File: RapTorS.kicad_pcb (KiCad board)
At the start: 2 copper layers, 22 parts, among them J1 Molex 48037-2200, J2 TestPoint, J3 TestPoint, J4 TestPoint, J5 TestPoint, J6 TestPoint, U1 PIC16LF1454-I_ML, U2 TLV71333PDBV, U3 E07-M1101S

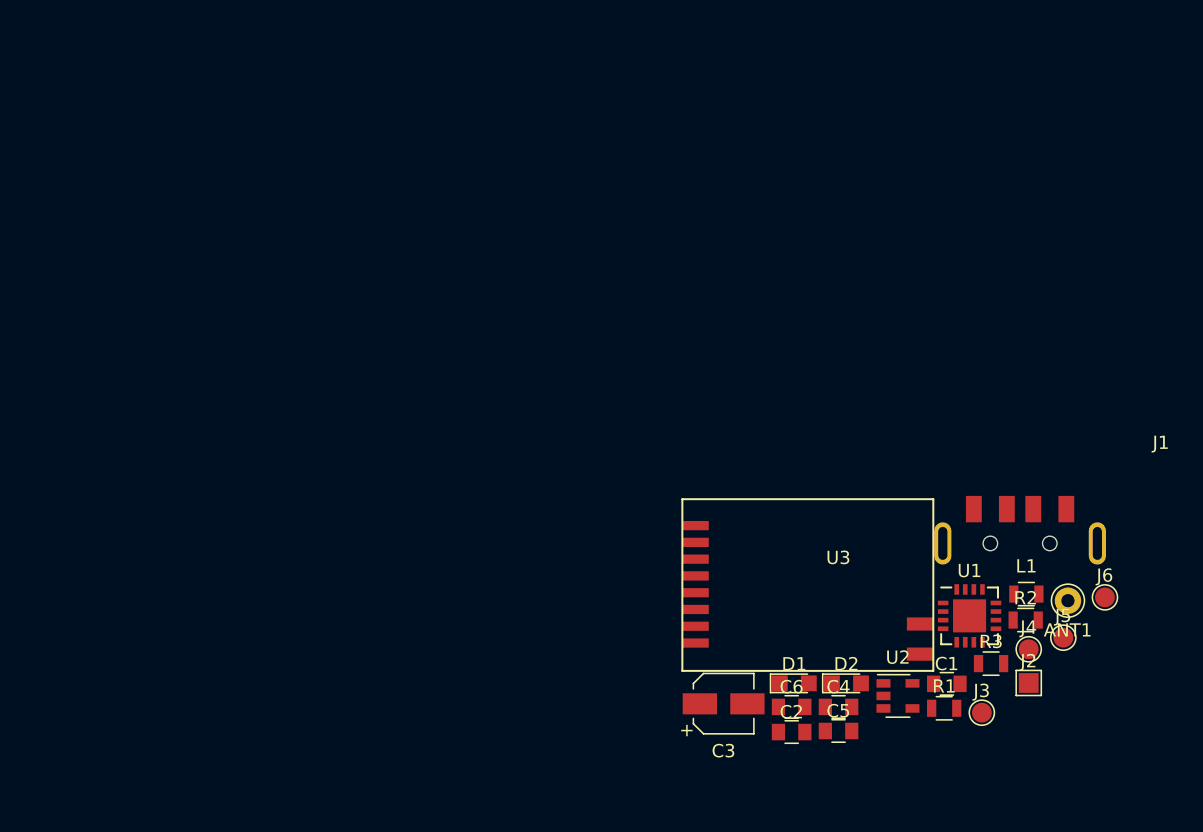
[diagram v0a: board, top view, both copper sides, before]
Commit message: first placement
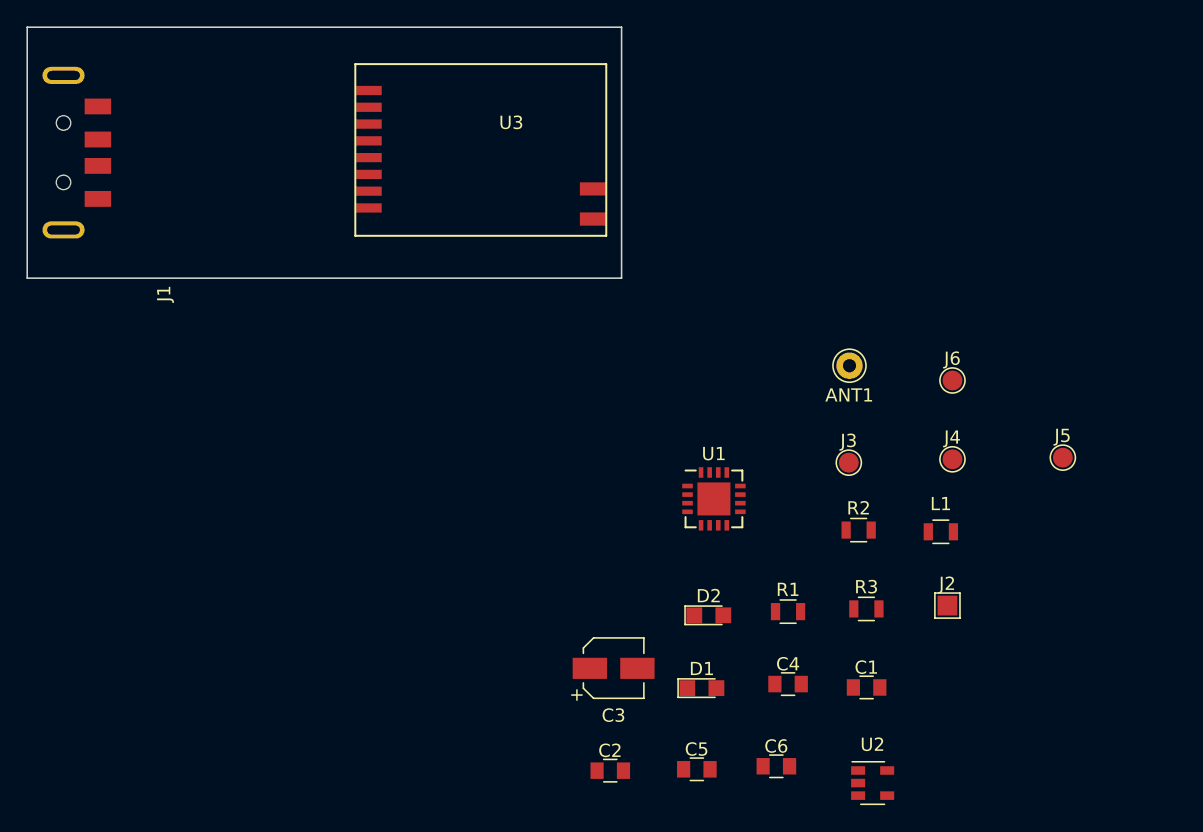
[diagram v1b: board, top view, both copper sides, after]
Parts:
- moved J1 78.2 mm to (2.75, 9.50), turned to 270 degrees
- moved U3 41.2 mm to (24.8, 2.79)
- moved ANT1 24.3 mm to (62.3, 25.6)
- moved J3 21.4 mm to (62.2, 33.0)
- moved U1 21.3 mm to (52.0, 35.7)
- moved J6 20.1 mm to (70.1, 26.7)
- moved J4 15.5 mm to (70.1, 32.7)
- moved R2 14.4 mm to (63.0, 38.1)
- moved C2 14.0 mm to (44.1, 56.3)
- moved R1 13.9 mm to (57.6, 44.2)
- moved J5 13.6 mm to (78.4, 32.6)
- moved D2 11.6 mm to (51.6, 44.5)
- moved C5 11.1 mm to (50.7, 56.2)
- moved R3 10.3 mm to (63.5, 44.0)
- moved C3 8.75 mm to (44.4, 48.5)
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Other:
- board outline added: 45 x 19 mm
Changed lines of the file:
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@@
   (general
     (thickness 1.6)
-    (drawings 0)
+    (drawings 4)
     (tracks 0)
     (zones 0)
@@
     (pad_to_mask_clearance 0.2)
     (aux_axis_origin 0 0)
-    (visible_elements FFFFFF7F)
+    (visible_elements FEFFF77F)
     (pcbplotparams
       (layerselection 0x010fc_ffffffff)
@@
   )
   (module Capacitors_SMD:CP_Elec_4x4.5 (layer F.Cu)
-    (at 52.727201 51.228801)
+    (at 44.3992 48.5394)
     (descr "SMT capacitor, aluminium electrolytic, 4x4.5")
     (attr smd)
@@
   )
   (module Capacitors_SMD:C_0805 (layer F.Cu)
-    (at 57.877201 51.463801)
+    (at 56.7182 55.9562)
     (descr "Capacitor SMD 0805, reflow soldering, AVX (see smccp.pdf)")
     (tags "capacitor 0805")
@@
   )
   (module Capacitors_SMD:C_0805 (layer F.Cu)
-    (at 61.427201 53.283801)
+    (at 50.6984 56.1848)
     (descr "Capacitor SMD 0805, reflow soldering, AVX (see smccp.pdf)")
     (tags "capacitor 0805")
@@
   )
   (module Capacitors_SMD:C_0805 (layer F.Cu)
-    (at 61.427201 51.463801)
+    (at 57.6072 49.7332)
     (descr "Capacitor SMD 0805, reflow soldering, AVX (see smccp.pdf)")
     (tags "capacitor 0805")
@@
   )
   (module Capacitors_SMD:C_0805 (layer F.Cu)
-    (at 57.877201 53.363801)
+    (at 44.1452 56.2864)
     (descr "Capacitor SMD 0805, reflow soldering, AVX (see smccp.pdf)")
     (tags "capacitor 0805")
@@
   )
   (module Capacitors_SMD:C_0805 (layer F.Cu)
-    (at 69.627201 49.713801)
+    (at 63.5508 49.9872)
     (descr "Capacitor SMD 0805, reflow soldering, AVX (see smccp.pdf)")
     (tags "capacitor 0805")
@@
   )
   (module Connectors:Pin_d1.0mm_L10.0mm (layer F.Cu)
-    (at 78.797201 43.418801)
+    (at 62.2554 25.6286)
     (descr "solder Pin_ diameter 1.0mm, hole diameter 1.0mm (press fit), length 10.0mm")
     (tags "solder Pin_ press fit")
@@
   )
   (module Connectors_TestPoints:Test_Point_Pad_1.5x1.5mm (layer F.Cu)
-    (at 75.827201 49.648801)
+    (at 69.6722 43.7896)
     (descr "SMD rectangular pad as test Point, square 1.5mm side length")
     (tags "test point SMD pad rectangle square")
@@
   )
   (module Connectors_TestPoints:Test_Point_Pad_d1.5mm (layer F.Cu)
-    (at 81.597201 43.168801)
+    (at 70.0532 26.7462)
     (descr "SMD pad as test Point, diameter 1.5mm")
     (tags "test point SMD pad")
@@
   )
   (module Connectors_TestPoints:Test_Point_Pad_d1.5mm (layer F.Cu)
-    (at 78.447201 46.218801)
+    (at 78.4098 32.5882)
     (descr "SMD pad as test Point, diameter 1.5mm")
     (tags "test point SMD pad")
@@
   )
   (module Connectors_TestPoints:Test_Point_Pad_d1.5mm (layer F.Cu)
-    (at 75.827201 47.098801)
+    (at 70.0532 32.7152)
     (descr "SMD pad as test Point, diameter 1.5mm")
     (tags "test point SMD pad")
@@
   )
   (module Connectors_TestPoints:Test_Point_Pad_d1.5mm (layer F.Cu)
-    (at 72.277201 51.898801)
+    (at 62.2046 32.9692)
     (descr "SMD pad as test Point, diameter 1.5mm")
     (tags "test point SMD pad")
@@
   )
   (module E07-M1101S:E07-M1101S (layer F.Cu)
-    (at 49.6022 35.7338)
+    (at 24.8412 2.794)
     (fp_text reference U3 (at 11.811 4.445) (layer F.SilkS)
       (effects (font (size 1 1) (thickness 0.15)))
@@
   )
   (module Housings_DFN_QFN:QFN-16-1EP_4x4mm_Pitch0.65mm (layer F.Cu)
-    (at 71.347201 44.568801)
+    (at 51.9938 35.7124)
     (descr "16-Lead Plastic Quad Flat, No Lead Package (ML) - 4x4x0.9 mm Body [QFN]; (see Microchip Packaging Specification 00000049BS.pdf)")
     (tags "QFN 0.65")
@@
   )
   (module Inductors_SMD:L_0805 (layer F.Cu)
-    (at 75.647201 42.918801)
+    (at 69.1744 38.2016)
     (descr "Resistor SMD 0805, reflow soldering, Vishay (see dcrcw.pdf)")
     (tags "resistor 0805")
@@
   )
   (module LEDs:LED_0805 (layer F.Cu)
-    (at 62.027201 49.678801)
+    (at 51.605 44.5262)
     (descr "LED 0805 smd package")
     (tags "LED led 0805 SMD smd SMT smt smdled SMDLED smtled SMTLED")
@@
   )
   (module LEDs:LED_0805 (layer F.Cu)
-    (at 58.077201 49.678801)
+    (at 51.0794 50.038)
     (descr "LED 0805 smd package")
     (tags "LED led 0805 SMD smd SMT smt smdled SMDLED smtled SMTLED")
@@
   )
   (module PX_Molex:MOLEX_USB_48037-2200 (layer F.Cu)
-    (at 75.1722 39.0838)
-    (attr smd)
-    (fp_text reference J1 (at 10.668 -7.62) (layer F.SilkS)
-      (effects (font (size 1 1) (thickness 0.15)))
-    )
-    (fp_text value "Molex 48037-2200" (at 3.556 -5.588) (layer F.Fab)
+    (at 2.75 9.5 270)
+    (attr smd)
+    (fp_text reference J1 (at 10.668 -7.62 270) (layer F.SilkS)
+      (effects (font (size 1 1) (thickness 0.15)))
+    )
+    (fp_text value "Molex 48037-2200" (at 3.556 -5.588 270) (layer F.Fab)
       (effects (font (size 1 1) (thickness 0.15)))
     )
     (fp_line (start -6 2.75) (end 6 2.75) (layer F.Fab) (width 0.12))
-    (pad 2 smd rect (at 1 -2.6) (size 1.2 2) (layers F.Cu F.Paste F.Mask)
+    (pad 2 smd rect (at 1 -2.6 270) (size 1.2 2) (layers F.Cu F.Paste F.Mask)
       (net 10 D-))
-    (pad 1 smd rect (at 3.5 -2.6) (size 1.2 2) (layers F.Cu F.Paste F.Mask)
+    (pad 1 smd rect (at 3.5 -2.6 270) (size 1.2 2) (layers F.Cu F.Paste F.Mask)
       (net 11 "Net-(C1-Pad1)"))
-    (pad 3 smd rect (at -1 -2.6) (size 1.2 2) (layers F.Cu F.Paste F.Mask)
+    (pad 3 smd rect (at -1 -2.6 270) (size 1.2 2) (layers F.Cu F.Paste F.Mask)
       (net 12 D+))
-    (pad 4 smd rect (at -3.5 -2.6) (size 1.2 2) (layers F.Cu F.Paste F.Mask)
-      (net 4 GND))
-    (pad "" np_thru_hole circle (at 2.25 0) (size 1.1 1.1) (drill 1.1) (layers *.Cu *.Mask))
-    (pad "" np_thru_hole circle (at -2.25 0) (size 1.1 1.1) (drill 1.1) (layers *.Cu *.Mask))
-    (pad 5 thru_hole roundrect (at -5.85 0) (size 1.3 3.2) (drill oval 0.7 2.5) (layers *.Cu *.Mask) (roundrect_rratio 0.5)
+    (pad 4 smd rect (at -3.5 -2.6 270) (size 1.2 2) (layers F.Cu F.Paste F.Mask)
+      (net 4 GND))
+    (pad "" np_thru_hole circle (at 2.25 0 270) (size 1.1 1.1) (drill 1.1) (layers *.Cu *.Mask))
+    (pad "" np_thru_hole circle (at -2.25 0 270) (size 1.1 1.1) (drill 1.1) (layers *.Cu *.Mask))
+    (pad 5 thru_hole roundrect (at -5.85 0 270) (size 1.3 3.2) (drill oval 0.7 2.5) (layers *.Cu *.Mask) (roundrect_rratio 0.5)
       (net 5 "Net-(J1-Pad5)"))
-    (pad 5 thru_hole roundrect (at 5.85 0) (size 1.3 3.2) (drill oval 0.7 2.5) (layers *.Cu *.Mask) (roundrect_rratio 0.5)
+    (pad 5 thru_hole roundrect (at 5.85 0 270) (size 1.3 3.2) (drill oval 0.7 2.5) (layers *.Cu *.Mask) (roundrect_rratio 0.5)
       (net 5 "Net-(J1-Pad5)"))
     (model "${KIPRJMOD}/3d_models/Molex 480372-200.step"
@@
   )
   (module Resistors_SMD:R_0805 (layer F.Cu)
-    (at 72.977201 48.183801)
+    (at 63.5356 44.0436)
     (descr "Resistor SMD 0805, reflow soldering, Vishay (see dcrcw.pdf)")
     (tags "resistor 0805")
@@
   )
   (module Resistors_SMD:R_0805 (layer F.Cu)
-    (at 75.597201 44.883801)
+    (at 62.9514 38.0746)
     (descr "Resistor SMD 0805, reflow soldering, Vishay (see dcrcw.pdf)")
     (tags "resistor 0805")
@@
   )
   (module Resistors_SMD:R_0805 (layer F.Cu)
-    (at 69.427201 51.563801)
+    (at 57.6072 44.2468)
     (descr "Resistor SMD 0805, reflow soldering, Vishay (see dcrcw.pdf)")
     (tags "resistor 0805")
@@
   )
   (module TO_SOT_Packages_SMD:SOT-23-5 (layer F.Cu)
-    (at 65.927201 50.628801)
+    (at 64.008 57.2262)
     (descr "5-pin SOT23 package")
     (tags SOT-23-5)
@@
     )
   )
+  (gr_line (start 0 0) (end 0 19) (layer Edge.Cuts) (width 0.12))
+  (gr_line (start 45 19) (end 0 19) (layer Edge.Cuts) (width 0.12))
+  (gr_line (start 45 0) (end 45 19) (layer Edge.Cuts) (width 0.12))
+  (gr_line (start 0 0) (end 45 0) (layer Edge.Cuts) (width 0.12))
 )

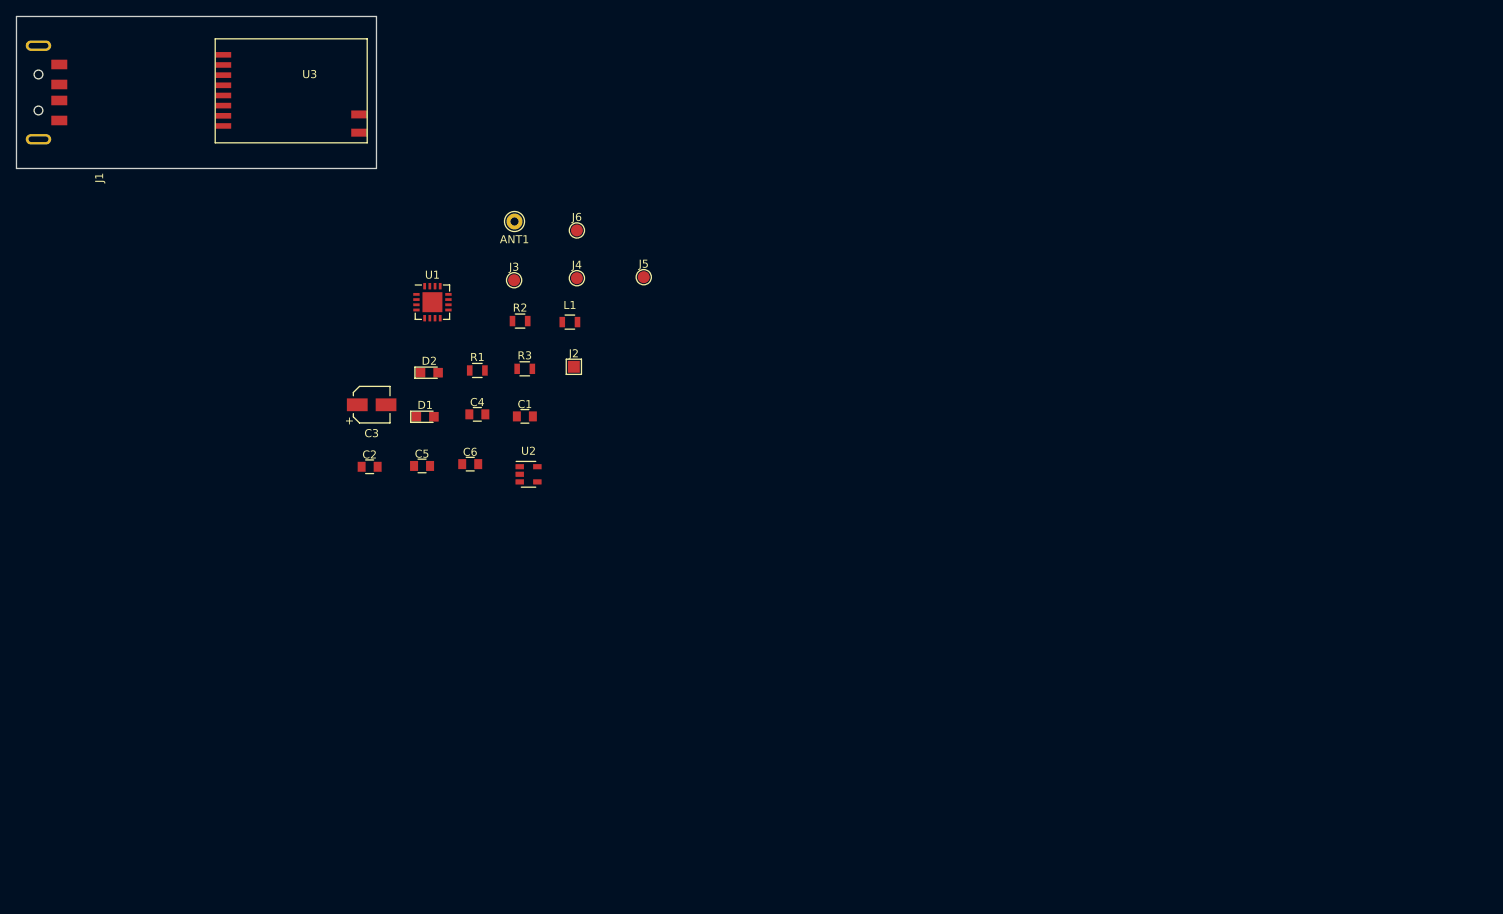
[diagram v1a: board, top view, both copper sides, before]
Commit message: placement second step
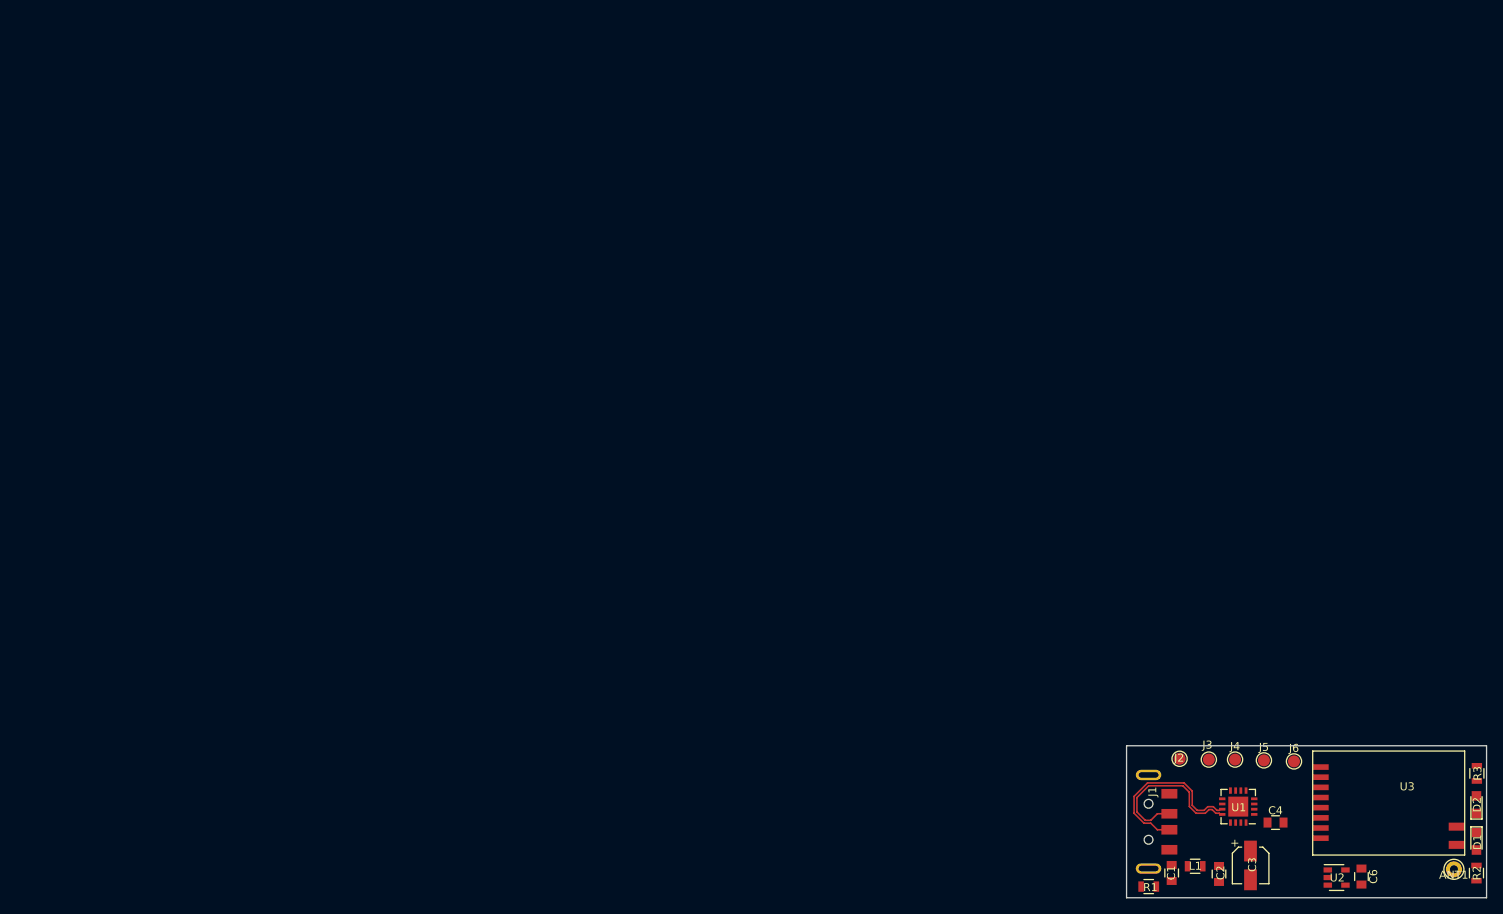
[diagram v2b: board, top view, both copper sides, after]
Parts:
- removed C5: 100nF, Capacitors_SMD:C_0805
- J2: footprint Connectors_TestPoints:Test_Point_Pad_1.5x1.5mm -> Connectors_TestPoints:Test_Point_Pad_d1.5mm
- moved J1 166.0 mm to (141.5, 100.7)
- moved U3 163.5 mm to (162.0, 91.8)
- moved ANT1 142.6 mm to (179.7, 106.6)
- moved D1 141.7 mm to (182.5, 103.1), turned to 270 degrees
- moved D2 141.6 mm to (182.5, 98.5), turned to 90 degrees
- moved R2 138.0 mm to (182.5, 107.1), turned to 90 degrees
- moved R3 129.3 mm to (182.5, 94.6), turned to 270 degrees
- moved C3 124.0 mm to (154.3, 106.1), turned to 270 degrees
- moved C6 122.8 mm to (168.1, 107.5), turned to 270 degrees
- moved U1 118.8 mm to (152.7, 98.8), turned to 180 degrees
- moved C2 117.7 mm to (150.3, 107.2), turned to 270 degrees
- moved U2 112.9 mm to (165.0, 107.6)
- moved C4 112.1 mm to (157.4, 100.8)
- moved J6 111.5 mm to (159.7, 93.1)
- moved R1 105.9 mm to (141.5, 108.8)
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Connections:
- U2 pad 4: Net-(U2-Pad4) -> (no net)
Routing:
- net D-: track 0.00 -> 22.0 mm
- net D+: track 0.00 -> 20.8 mm
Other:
- net class Default: clearance 0.2 -> 0.16
- rule trace_clearance: 0.2 -> 0.16
- rule trace_min: 0.2 -> 0.16
